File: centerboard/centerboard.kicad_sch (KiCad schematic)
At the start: 12 parts, among them J1 Conn_01x10_MountingPin, U1 ProMicro

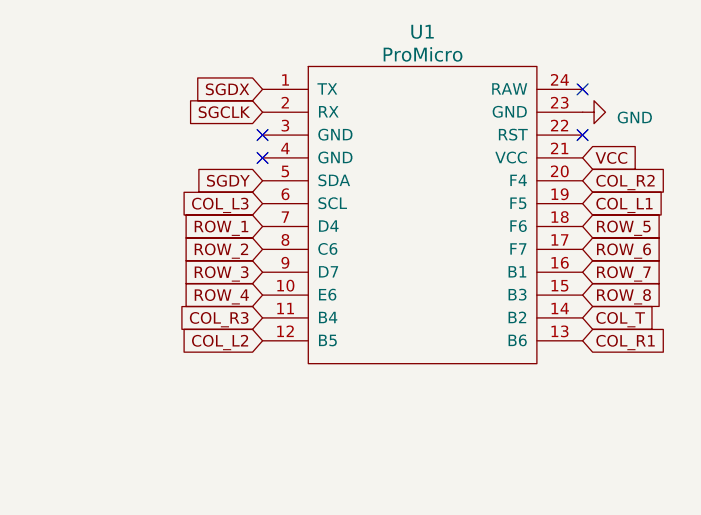
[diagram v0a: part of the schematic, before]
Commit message: redo centerboard again (and again)
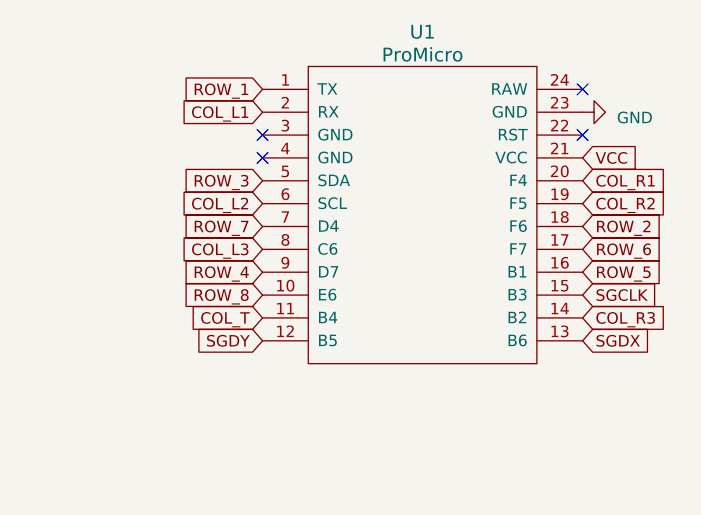
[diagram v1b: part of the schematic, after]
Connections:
- net COL_L1: now also U1.2 (RX); no longer U1.19 (F5)
- net COL_L2: now also U1.6 (SCL); no longer U1.12 (B5)
- net COL_L3: now also U1.8 (C6); no longer U1.6 (SCL)
- net COL_R1: now also U1.20 (F4); no longer U1.13 (B6)
- net COL_R2: now also U1.19 (F5); no longer U1.20 (F4)
- net COL_R3: now also U1.14 (B2); no longer U1.11 (B4)
- net COL_T: now also U1.11 (B4); no longer U1.14 (B2)
- net ROW_1: now also U1.1 (TX); no longer U1.7 (D4)
- net ROW_2: now also U1.18 (F6); no longer U1.8 (C6)
- net ROW_3: now also U1.5 (SDA); no longer U1.9 (D7)
- net ROW_4: now also U1.9 (D7); no longer U1.10 (E6)
- net ROW_5: now also U1.16 (B1); no longer U1.18 (F6)
- net ROW_7: now also U1.7 (D4); no longer U1.16 (B1)
- net ROW_8: now also U1.10 (E6); no longer U1.15 (B3)
- net SGCLK: now also U1.15 (B3); no longer U1.2 (RX)
- net SGDX: now also U1.13 (B6); no longer U1.1 (TX)
- net SGDY: now also U1.12 (B5); no longer U1.5 (SDA)
